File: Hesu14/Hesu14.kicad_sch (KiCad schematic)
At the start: 34 parts, among them J2 OLED_128x32, U1 RP2040_Zero

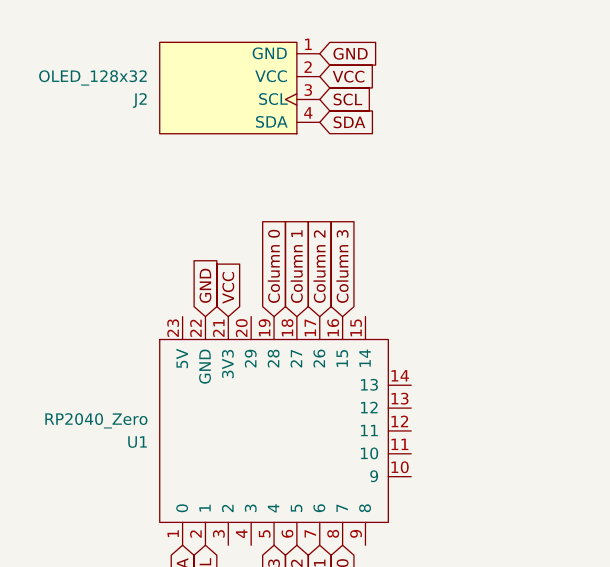
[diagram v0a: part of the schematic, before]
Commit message: Update PCB and Case
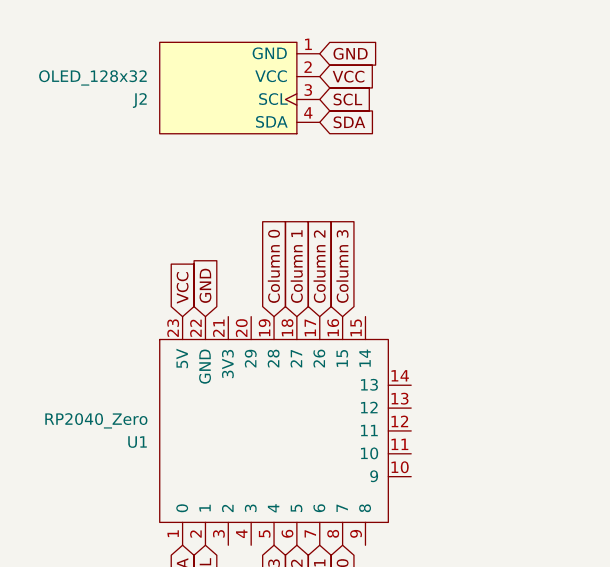
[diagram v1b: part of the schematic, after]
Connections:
- net VCC: now also U1.23 (5V); no longer U1.21 (3V3)
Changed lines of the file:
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@@
 	(global_label "VCC"
 		(shape input)
-		(at 93.98 82.55 90)
+		(at 88.9 82.55 90)
 		(fields_autoplaced yes)
 		(effects
@@
 		)
 		(property "Intersheetrefs" "${INTERSHEET_REFS}"
-			(at 93.98 75.9362 90)
+			(at 88.9 75.9362 90)
 			(effects
 				(font
